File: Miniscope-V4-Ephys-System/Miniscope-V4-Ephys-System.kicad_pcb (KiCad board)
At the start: 4 copper layers, 36.1 x 27.2 mm, 67 parts, among them J1 34 Circuit Slimslack Connector, J10 Conn_01x01, J11 Conn_01x01, J12 Conn_01x01, J13 Conn_01x01, J14 Conn_01x05, J15 Conn_01x01, J16 Conn_01x01, J17 Conn_01x01, J18 Conn_01x01, J19 Conn_01x01, J2 Conn_01x01, J20 Conn_01x01, J21 Conn_01x01, J22 Conn_01x01, J23 Conn_01x01, J24 Conn_01x01, J25 Conn_01x01, J26 Conn_01x01, J27 Conn_01x01, J28 Conn_01x01, J3 Conn_01x01, J4 Conn_01x01, J5 Conn_01x01, J6 Conn_01x01, J7 Conn_01x01, J8 Conn_01x01, J9 Conn_01x01, Q1 MMBT3904LP-7B, U1 RHD2132, U2 TXB0304RUT, U3 MCP1711T-30I/5X, U4 ATSAME70N21A-CN, U5 MCP1711T-18I/5X, Y1 SMD_CRYSTAL

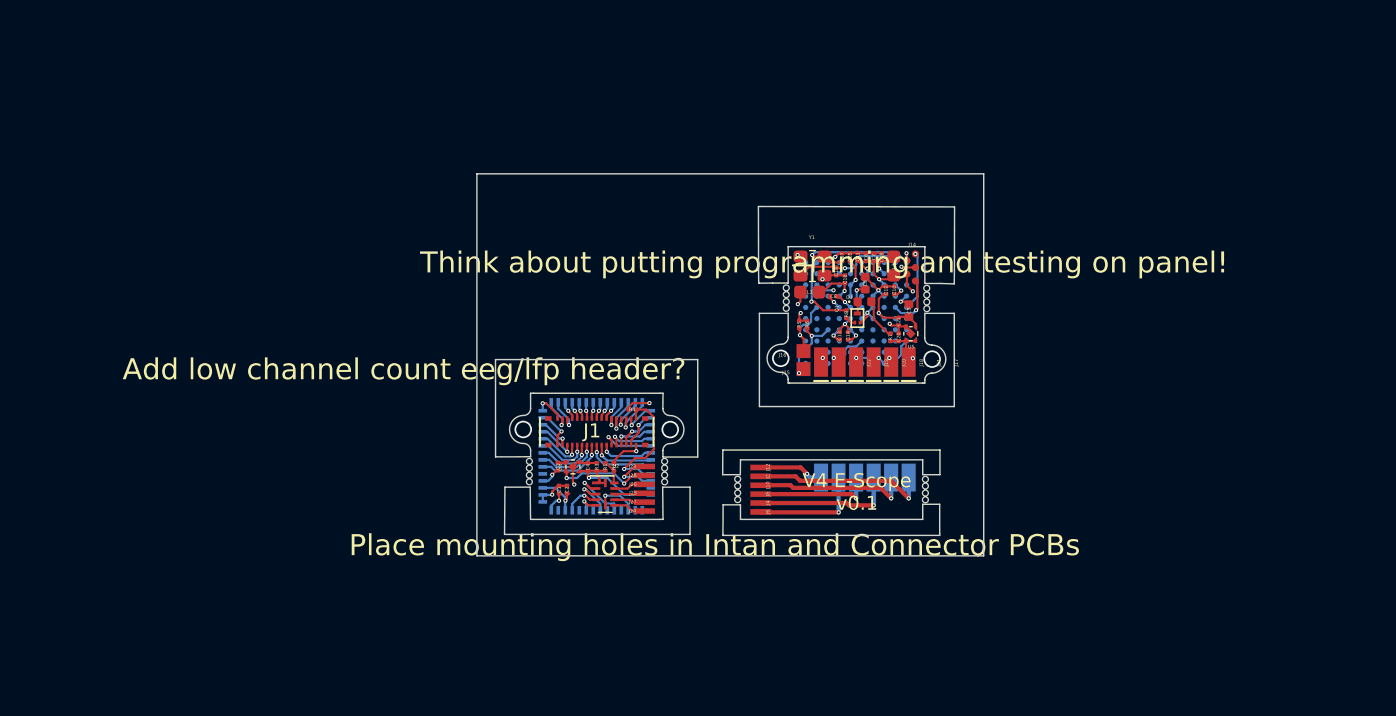
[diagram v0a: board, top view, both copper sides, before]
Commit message: Add files via upload
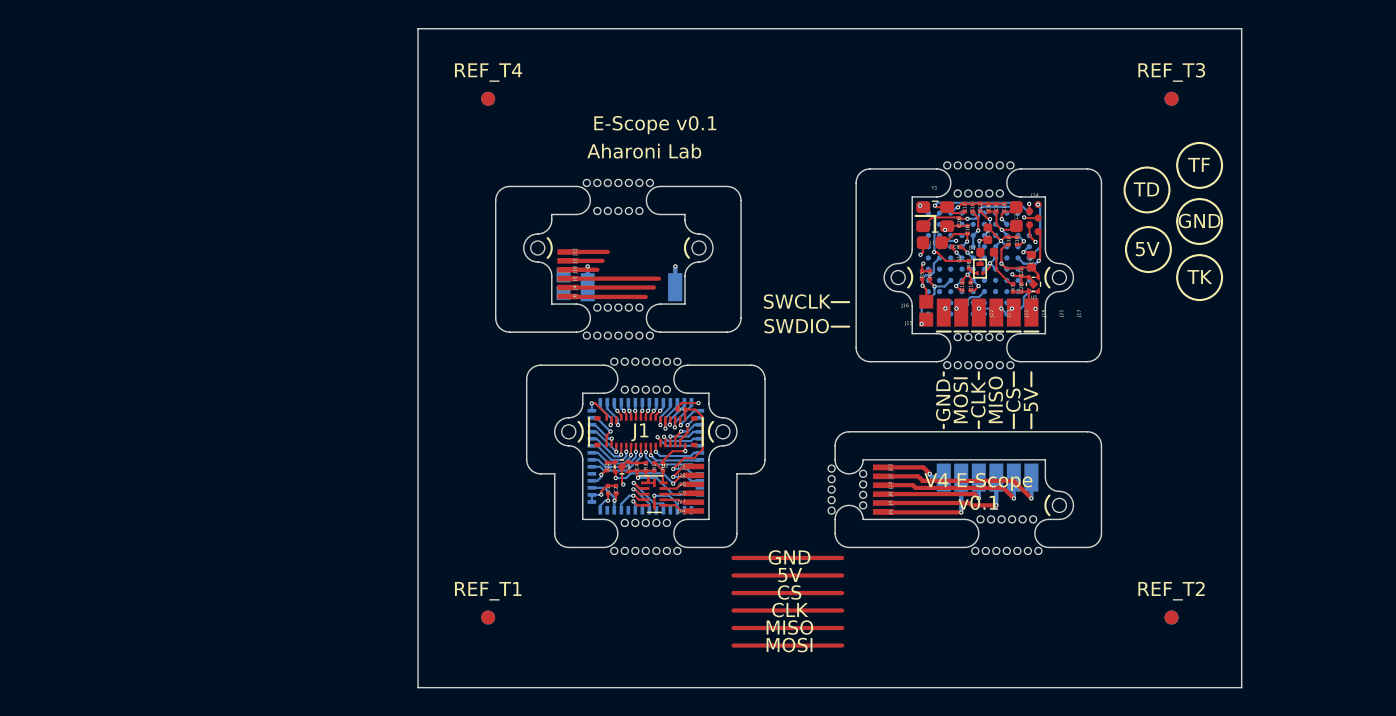
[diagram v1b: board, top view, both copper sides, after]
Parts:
- removed the J10 at (119.5, 132.6)
- removed the J12 at (119.5, 131.3)
- removed the J13 at (123.8, 132.0)
- removed the J2 at (119.5, 131.9)
- removed the J3 at (130.0, 132.0)
- removed the J4 at (119.5, 133.8)
- removed the J6 at (119.5, 134.5)
- removed the J8 at (119.5, 133.2)
- added HOLE: Conn_1x1_700_Circular_Pad, .Connector:Conn_1x1_700_Circular_Pad, F.Cu at (107.8, 119.9)
- added HOLE: Conn_1x1_700_Circular_Pad, .Connector:Conn_1x1_700_Circular_Pad, F.Cu at (110.8, 111.0)
- added HOLE: Conn_1x1_700_Circular_Pad, .Connector:Conn_1x1_700_Circular_Pad, F.Cu at (140.8, 117.8)
- added HOLE: Conn_1x1_700_Circular_Pad, .Connector:Conn_1x1_700_Circular_Pad, F.Cu at (129.2, 117.8)
- added HOLE: Conn_1x1_700_Circular_Pad, .Connector:Conn_1x1_700_Circular_Pad, F.Cu at (110.0, 113.0)
- added HOLE: Conn_1x1_700_Circular_Pad, .Connector:Conn_1x1_700_Circular_Pad, F.Cu at (109.3, 113.0)
- added HOLE: Conn_1x1_700_Circular_Pad, .Connector:Conn_1x1_700_Circular_Pad, F.Cu at (109.3, 111.0)
- added HOLE: Conn_1x1_700_Circular_Pad, .Connector:Conn_1x1_700_Circular_Pad, F.Cu at (107.8, 111.0)
- added HOLE: Conn_1x1_700_Circular_Pad, .Connector:Conn_1x1_700_Circular_Pad, F.Cu at (108.5, 111.0)
- added HOLE: Conn_1x1_700_Circular_Pad, .Connector:Conn_1x1_700_Circular_Pad, F.Cu at (107.8, 113.0)
- added HOLE: Conn_1x1_700_Circular_Pad, .Connector:Conn_1x1_700_Circular_Pad, F.Cu at (110.8, 113.0)
- added HOLE: Conn_1x1_700_Circular_Pad, .Connector:Conn_1x1_700_Circular_Pad, F.Cu at (110.0, 111.0)
- added HOLE: Conn_1x1_700_Circular_Pad, .Connector:Conn_1x1_700_Circular_Pad, F.Cu at (108.5, 113.0)
- added HOLE: Conn_1x1_700_Circular_Pad, .Connector:Conn_1x1_700_Circular_Pad, F.Cu at (108.5, 121.9)
- added HOLE: Conn_1x1_700_Circular_Pad, .Connector:Conn_1x1_700_Circular_Pad, F.Cu at (107.8, 121.9)
- added HOLE: Conn_1x1_700_Circular_Pad, .Connector:Conn_1x1_700_Circular_Pad, F.Cu at (108.5, 119.9)
- added HOLE: Conn_1x1_700_Circular_Pad, .Connector:Conn_1x1_700_Circular_Pad, F.Cu at (109.3, 119.9)
- added HOLE: Conn_1x1_700_Circular_Pad, .Connector:Conn_1x1_700_Circular_Pad, F.Cu at (109.3, 121.9)
- added HOLE: Conn_1x1_700_Circular_Pad, .Connector:Conn_1x1_700_Circular_Pad, F.Cu at (110.8, 121.9)
- added HOLE: Conn_1x1_700_Circular_Pad, .Connector:Conn_1x1_700_Circular_Pad, F.Cu at (110.0, 121.9)
- added HOLE: Conn_1x1_700_Circular_Pad, .Connector:Conn_1x1_700_Circular_Pad, F.Cu at (110.8, 119.9)
- added HOLE: Conn_1x1_700_Circular_Pad, .Connector:Conn_1x1_700_Circular_Pad, F.Cu at (138.9, 135.0)
- added HOLE: Conn_1x1_700_Circular_Pad, .Connector:Conn_1x1_700_Circular_Pad, F.Cu at (139.2, 137.2)
- added HOLE: Conn_1x1_700_Circular_Pad, .Connector:Conn_1x1_700_Circular_Pad, F.Cu at (134.8, 137.2)
- added HOLE: Conn_1x1_700_Circular_Pad, .Connector:Conn_1x1_700_Circular_Pad, F.Cu at (110.0, 119.9)
- added HOLE: Conn_1x1_700_Circular_Pad, .Connector:Conn_1x1_700_Circular_Pad, F.Cu at (137.4, 135.0)
- added HOLE: Conn_1x1_700_Circular_Pad, .Connector:Conn_1x1_700_Circular_Pad, F.Cu at (136.2, 137.2)
- added HOLE: Conn_1x1_700_Circular_Pad, .Connector:Conn_1x1_700_Circular_Pad, F.Cu at (135.1, 135.0)
- added HOLE: Conn_1x1_700_Circular_Pad, .Connector:Conn_1x1_700_Circular_Pad, F.Cu at (138.1, 135.0)
- added HOLE: Conn_1x1_700_Circular_Pad, .Connector:Conn_1x1_700_Circular_Pad, F.Cu at (137.8, 137.2)
- added HOLE: Conn_1x1_700_Circular_Pad, .Connector:Conn_1x1_700_Circular_Pad, F.Cu at (138.5, 137.2)
- added HOLE: Conn_1x1_700_Circular_Pad, .Connector:Conn_1x1_700_Circular_Pad, F.Cu at (137.0, 137.2)
- added HOLE: Conn_1x1_700_Circular_Pad, .Connector:Conn_1x1_700_Circular_Pad, F.Cu at (136.6, 135.0)
- added HOLE: Conn_1x1_700_Circular_Pad, .Connector:Conn_1x1_700_Circular_Pad, F.Cu at (135.9, 135.0)
- added HOLE: Conn_1x1_700_Circular_Pad, .Connector:Conn_1x1_700_Circular_Pad, F.Cu at (135.5, 137.2)
- added HOLE: Conn_1x1_700_Circular_Pad, .Connector:Conn_1x1_700_Circular_Pad, F.Cu at (107.0, 121.9)
- added HOLE: Conn_1x1_700_Circular_Pad, .Connector:Conn_1x1_700_Circular_Pad, F.Cu at (124.5, 131.4)
- added HOLE: Conn_1x1_700_Circular_Pad, .Connector:Conn_1x1_700_Circular_Pad, F.Cu at (124.5, 134.4)
- added HOLE: Conn_1x1_700_Circular_Pad, .Connector:Conn_1x1_700_Circular_Pad, F.Cu at (126.8, 131.8)
- added HOLE: Conn_1x1_700_Circular_Pad, .Connector:Conn_1x1_700_Circular_Pad, F.Cu at (113.5, 137.2)
- added HOLE: Conn_1x1_700_Circular_Pad, .Connector:Conn_1x1_700_Circular_Pad, F.Cu at (109.0, 137.2)
- added HOLE: Conn_1x1_700_Circular_Pad, .Connector:Conn_1x1_700_Circular_Pad, F.Cu at (109.0, 123.8)
- added HOLE: Conn_1x1_700_Circular_Pad, .Connector:Conn_1x1_700_Circular_Pad, F.Cu at (113.5, 123.8)
- added HOLE: Conn_1x1_700_Circular_Pad, .Connector:Conn_1x1_700_Circular_Pad, F.Cu at (132.8, 109.8)
- added HOLE: Conn_1x1_700_Circular_Pad, .Connector:Conn_1x1_700_Circular_Pad, F.Cu at (137.2, 109.8)
- added HOLE: Conn_1x1_700_Circular_Pad, .Connector:Conn_1x1_700_Circular_Pad, F.Cu at (137.2, 124.0)
- added HOLE: Conn_1x1_700_Circular_Pad, .Connector:Conn_1x1_700_Circular_Pad, F.Cu at (111.5, 121.9)
- added HOLE: Conn_1x1_700_Circular_Pad, .Connector:Conn_1x1_700_Circular_Pad, F.Cu at (132.8, 124.0)
- added HOLE: Conn_1x1_700_Circular_Pad, .Connector:Conn_1x1_700_Circular_Pad, F.Cu at (124.5, 132.9)
- added HOLE: Conn_1x1_700_Circular_Pad, .Connector:Conn_1x1_700_Circular_Pad, F.Cu at (126.8, 132.5)
- added HOLE: Conn_1x1_700_Circular_Pad, .Connector:Conn_1x1_700_Circular_Pad, F.Cu at (124.5, 133.6)
- added HOLE: Conn_1x1_700_Circular_Pad, .Connector:Conn_1x1_700_Circular_Pad, F.Cu at (126.8, 134.0)
- added HOLE: Conn_1x1_700_Circular_Pad, .Connector:Conn_1x1_700_Circular_Pad, F.Cu at (126.8, 133.2)
- added HOLE: Conn_1x1_700_Circular_Pad, .Connector:Conn_1x1_700_Circular_Pad, F.Cu at (124.5, 132.1)
- added HOLE: Conn_1x1_700_Circular_Pad, .Connector:Conn_1x1_700_Circular_Pad, F.Cu at (135.8, 122.0)
- added HOLE: Conn_1x1_700_Circular_Pad, .Connector:Conn_1x1_700_Circular_Pad, F.Cu at (134.2, 124.0)
- added HOLE: Conn_1x1_700_Circular_Pad, .Connector:Conn_1x1_700_Circular_Pad, F.Cu at (133.5, 122.0)
- added HOLE: Conn_1x1_700_Circular_Pad, .Connector:Conn_1x1_700_Circular_Pad, F.Cu at (111.5, 111.0)
- added HOLE: Conn_1x1_700_Circular_Pad, .Connector:Conn_1x1_700_Circular_Pad, F.Cu at (136.5, 122.0)
- added HOLE: Conn_1x1_700_Circular_Pad, .Connector:Conn_1x1_700_Circular_Pad, F.Cu at (135.8, 124.0)
- added HOLE: Conn_1x1_700_Circular_Pad, .Connector:Conn_1x1_700_Circular_Pad, F.Cu at (136.5, 124.0)
- added HOLE: Conn_1x1_700_Circular_Pad, .Connector:Conn_1x1_700_Circular_Pad, F.Cu at (135.0, 124.0)
- added HOLE: Conn_1x1_700_Circular_Pad, .Connector:Conn_1x1_700_Circular_Pad, F.Cu at (135.0, 122.0)
- added HOLE: Conn_1x1_700_Circular_Pad, .Connector:Conn_1x1_700_Circular_Pad, F.Cu at (134.2, 122.0)
- added HOLE: Conn_1x1_700_Circular_Pad, .Connector:Conn_1x1_700_Circular_Pad, F.Cu at (133.5, 124.0)
- added HOLE: Conn_1x1_700_Circular_Pad, .Connector:Conn_1x1_700_Circular_Pad, F.Cu at (134.2, 111.8)
- added HOLE: Conn_1x1_700_Circular_Pad, .Connector:Conn_1x1_700_Circular_Pad, F.Cu at (135.8, 109.8)
- added HOLE: Conn_1x1_700_Circular_Pad, .Connector:Conn_1x1_700_Circular_Pad, F.Cu at (136.5, 111.8)
- added HOLE: Conn_1x1_700_Circular_Pad, .Connector:Conn_1x1_700_Circular_Pad, F.Cu at (107.0, 111.0)
- added HOLE: Conn_1x1_700_Circular_Pad, .Connector:Conn_1x1_700_Circular_Pad, F.Cu at (133.5, 111.8)
- added HOLE: Conn_1x1_700_Circular_Pad, .Connector:Conn_1x1_700_Circular_Pad, F.Cu at (134.2, 109.8)
- added HOLE: Conn_1x1_700_Circular_Pad, .Connector:Conn_1x1_700_Circular_Pad, F.Cu at (133.5, 109.8)
- added HOLE: Conn_1x1_700_Circular_Pad, .Connector:Conn_1x1_700_Circular_Pad, F.Cu at (135.0, 109.8)
- added HOLE: Conn_1x1_700_Circular_Pad, .Connector:Conn_1x1_700_Circular_Pad, F.Cu at (135.0, 111.8)
- added HOLE: Conn_1x1_700_Circular_Pad, .Connector:Conn_1x1_700_Circular_Pad, F.Cu at (135.8, 111.8)
- added HOLE: Conn_1x1_700_Circular_Pad, .Connector:Conn_1x1_700_Circular_Pad, F.Cu at (136.5, 109.8)
- added HOLE: Conn_1x1_700_Circular_Pad, .Connector:Conn_1x1_700_Circular_Pad, F.Cu at (110.5, 123.8)
- added HOLE: Conn_1x1_700_Circular_Pad, .Connector:Conn_1x1_700_Circular_Pad, F.Cu at (109.8, 123.8)
- added HOLE: Conn_1x1_700_Circular_Pad, .Connector:Conn_1x1_700_Circular_Pad, F.Cu at (112.0, 123.8)
- added HOLE: Conn_1x1_700_Circular_Pad, .Connector:Conn_1x1_700_Circular_Pad, F.Cu at (103.5, 115.6)
- added HOLE: Conn_1x1_700_Circular_Pad, .Connector:Conn_1x1_700_Circular_Pad, F.Cu at (112.8, 123.8)
- added HOLE: Conn_1x1_700_Circular_Pad, .Connector:Conn_1x1_700_Circular_Pad, F.Cu at (111.2, 123.8)
- added HOLE: Conn_1x1_700_Circular_Pad, .Connector:Conn_1x1_700_Circular_Pad, F.Cu at (110.5, 125.8)
- added HOLE: Conn_1x1_700_Circular_Pad, .Connector:Conn_1x1_700_Circular_Pad, F.Cu at (109.8, 125.8)
- added HOLE: Conn_1x1_700_Circular_Pad, .Connector:Conn_1x1_700_Circular_Pad, F.Cu at (112.0, 125.8)
- added HOLE: Conn_1x1_700_Circular_Pad, .Connector:Conn_1x1_700_Circular_Pad, F.Cu at (112.8, 125.8)
- added HOLE: Conn_1x1_700_Circular_Pad, .Connector:Conn_1x1_700_Circular_Pad, F.Cu at (111.2, 125.8)
- added HOLE: Conn_1x1_700_Circular_Pad, .Connector:Conn_1x1_700_Circular_Pad, F.Cu at (110.5, 137.2)
- added HOLE: Conn_1x1_700_Circular_Pad, .Connector:Conn_1x1_700_Circular_Pad, F.Cu at (109.8, 137.2)
- added HOLE: Conn_1x1_700_Circular_Pad, .Connector:Conn_1x1_700_Circular_Pad, F.Cu at (112.0, 137.2)
- added HOLE: Conn_1x1_700_Circular_Pad, .Connector:Conn_1x1_700_Circular_Pad, F.Cu at (115.0, 115.6)
- added HOLE: Conn_1x1_700_Circular_Pad, .Connector:Conn_1x1_700_Circular_Pad, F.Cu at (112.8, 137.2)
- added HOLE: Conn_1x1_700_Circular_Pad, .Connector:Conn_1x1_700_Circular_Pad, F.Cu at (111.2, 137.2)
- added HOLE: Conn_1x1_700_Circular_Pad, .Connector:Conn_1x1_700_Circular_Pad, F.Cu at (112.8, 135.2)
- added HOLE: Conn_1x1_700_Circular_Pad, .Connector:Conn_1x1_700_Circular_Pad, F.Cu at (112.0, 135.2)
- added HOLE: Conn_1x1_700_Circular_Pad, .Connector:Conn_1x1_700_Circular_Pad, F.Cu at (111.2, 135.2)
- added HOLE: Conn_1x1_700_Circular_Pad, .Connector:Conn_1x1_700_Circular_Pad, F.Cu at (110.5, 135.2)
- added HOLE: Conn_1x1_700_Circular_Pad, .Connector:Conn_1x1_700_Circular_Pad, F.Cu at (109.8, 135.2)
- added HOLE: Conn_1x1_700_Circular_Pad, .Connector:Conn_1x1_700_Circular_Pad, F.Cu at (140.8, 134.0)
- added HOLE: Conn_1x1_700_Circular_Pad, .Connector:Conn_1x1_700_Circular_Pad, F.Cu at (105.8, 128.8)
- added HOLE: Conn_1x1_700_Circular_Pad, .Connector:Conn_1x1_700_Circular_Pad, F.Cu at (116.8, 128.8)
- added J10: Conn_01x01, .Connector:Conn_1x1_250x750_Pad, F.Cu at (105.7, 117.2)
- added J10: Conn_01x01, .Connector:Conn_1x1_250x750_Pad, F.Cu at (128.2, 132.6)
- added J12: Conn_01x01, .Connector:Conn_1x1_250x750_Pad, F.Cu at (105.7, 115.9)
- added J12: Conn_01x01, .Connector:Conn_1x1_250x750_Pad, F.Cu at (128.2, 131.3)
- added J13: Conn_01x01, .Connector:Conn_1x1_250x750_Pad, B.Cu at (113.3, 118.4)
- added J13: Conn_01x01, .Connector:Conn_1x1_250x750_Pad, B.Cu at (132.5, 132.0)
- added J2: Conn_01x01, .Connector:Conn_1x1_250x750_Pad, F.Cu at (105.7, 116.6)
- added J2: Conn_01x01, .Connector:Conn_1x1_250x750_Pad, F.Cu at (128.2, 131.9)
- added J3: Conn_01x01, .Connector:Conn_1x1_250x750_Pad, B.Cu at (105.4, 118.9)
- added J3: Conn_01x01, .Connector:Conn_1x1_250x750_Pad, B.Cu at (105.4, 117.6)
- added J3: Conn_01x01, .Connector:Conn_1x1_250x750_Pad, B.Cu at (107.1, 118.4)
- added J3: Conn_01x01, .Connector:Conn_1x1_250x750_Pad, B.Cu at (138.8, 132.0)
- added J4: Conn_01x01, .Connector:Conn_1x1_250x750_Pad, F.Cu at (105.7, 118.5)
- added J4: Conn_01x01, .Connector:Conn_1x1_250x750_Pad, F.Cu at (128.2, 133.8)
- added J6: Conn_01x01, .Connector:Conn_1x1_250x750_Pad, F.Cu at (105.7, 119.1)
- added J6: Conn_01x01, .Connector:Conn_1x1_250x750_Pad, F.Cu at (128.2, 134.5)
- added J8: Conn_01x01, .Connector:Conn_1x1_250x750_Pad, F.Cu at (105.7, 117.8)
- added J8: Conn_01x01, .Connector:Conn_1x1_250x750_Pad, F.Cu at (128.2, 133.2)
- added REF_B1: Fiducial_1mm_Mask2mm, Fiducial:Fiducial_1mm_Mask2mm, B.Cu at (100.0, 142.0)
- added REF_B2: Fiducial_1mm_Mask2mm, Fiducial:Fiducial_1mm_Mask2mm, B.Cu at (148.8, 142.0)
- added REF_B3: Fiducial_1mm_Mask2mm, Fiducial:Fiducial_1mm_Mask2mm, B.Cu at (148.8, 105.0)
- added REF_B4: Fiducial_1mm_Mask2mm, Fiducial:Fiducial_1mm_Mask2mm, B.Cu at (100.0, 105.0)
- added REF_T1: Fiducial_1mm_Mask2mm, Fiducial:Fiducial_1mm_Mask2mm, F.Cu at (100.0, 142.0)
- added REF_T2: Fiducial_1mm_Mask2mm, Fiducial:Fiducial_1mm_Mask2mm, F.Cu at (148.8, 142.0)
- added REF_T3: Fiducial_1mm_Mask2mm, Fiducial:Fiducial_1mm_Mask2mm, F.Cu at (148.8, 105.0)
- added REF_T4: Fiducial_1mm_Mask2mm, Fiducial:Fiducial_1mm_Mask2mm, F.Cu at (100.0, 105.0)
- moved C11 9.43 mm to (135.1, 112.7)
- moved C16 9.43 mm to (133.6, 113.8)
- moved C5 9.43 mm to (135.6, 114.6)
- moved C13 9.43 mm to (133.8, 118.4)
- moved C14 9.43 mm to (134.4, 118.4)
- moved C18 9.43 mm to (134.2, 114.3)
- moved C7 9.43 mm to (136.3, 112.8)
- moved C20 9.43 mm to (138.0, 118.5)
- moved C21 9.43 mm to (138.0, 117.4)
- moved J15 9.43 mm to (131.2, 120.8)
- moved J16 9.43 mm to (131.2, 119.5)
- moved J17 9.43 mm to (138.8, 120.2)
- moved J18 9.43 mm to (136.2, 120.2)
- moved J19 9.43 mm to (133.8, 120.2)
- moved J20 9.43 mm to (135.0, 120.2)
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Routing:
- net (no net): track 0.00 -> 28.6 mm, vias 4 -> 2
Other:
- board size 36.1 x 27.2 mm -> 58.8 x 47 mm
- board text added: "5V"
- board text added: "Aharoni Lab"
- board text added: "CLK"
- board text added: "CS"
- board text added: "E-Scope v0.1"
- board text added: "GND"
- board text added: "MISO"
- board text added: "MOSI"
- board text added: "SWCLK"
- board text added: "SWDIO"
- board text added: "TD"
- board text added: "TF"
- board text added: "TK"
- board text removed: "Add low channel count eeg/lfp header?"
- board text removed: "Place mounting holes in Intan and Connector PCBs"
- board text removed: "Think about putting programming and testing on panel!"
